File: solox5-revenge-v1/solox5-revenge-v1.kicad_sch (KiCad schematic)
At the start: 36 parts, among them J1 AudioJack4, J2 USB_B_Micro, J3 USB_A, J4 Micro_SD_Card_Det1, SW1 SW_SPDT_MSM, U1 LTC4054ES5-4.2, U2 MIX2018A, U3 AC6965E

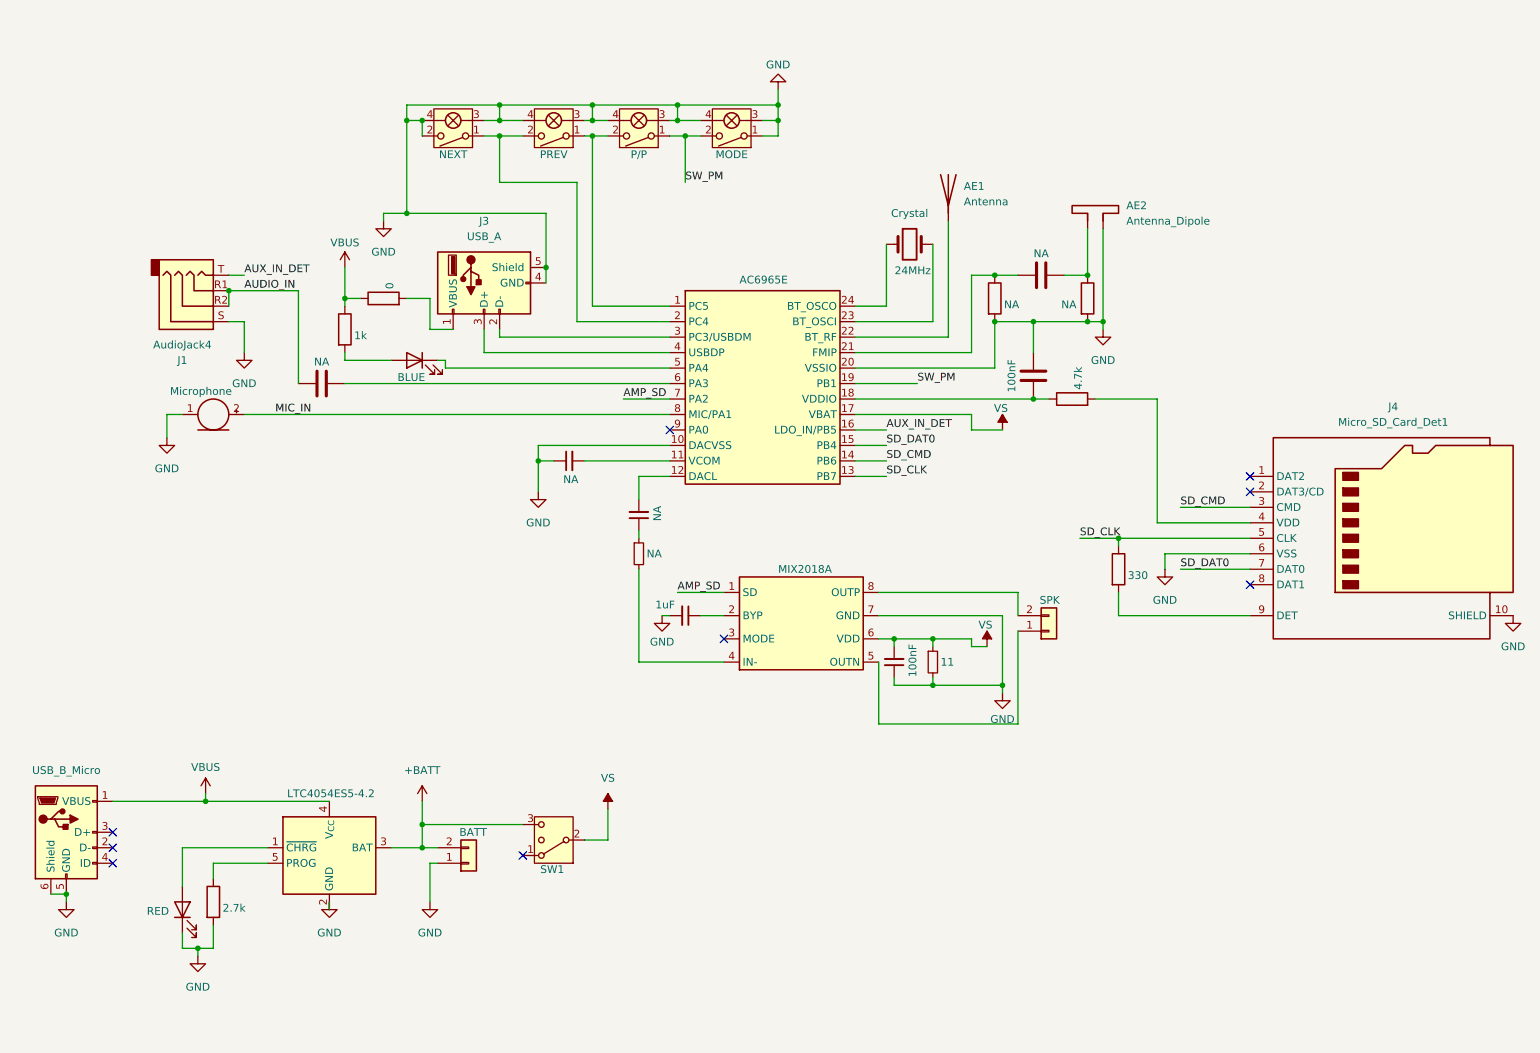
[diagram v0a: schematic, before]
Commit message: [KICAD] Update Sources
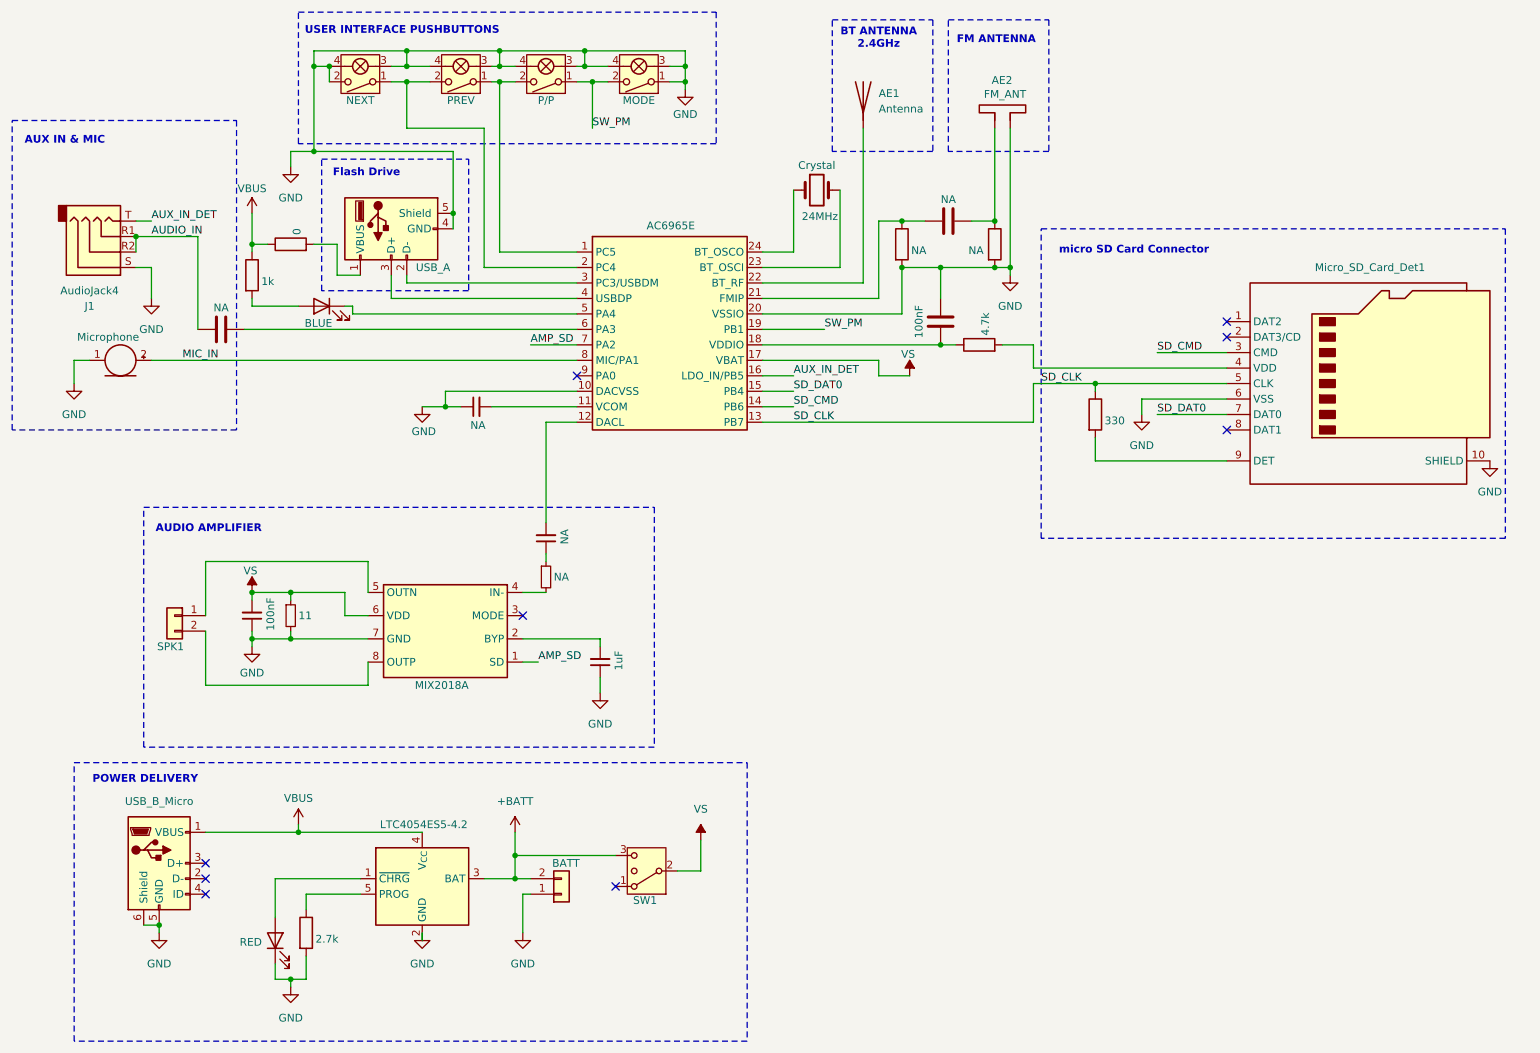
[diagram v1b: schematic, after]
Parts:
- removed C6: 100nF, symbol Device:C_Small
- removed R9: 11, symbol Device:R_Small
- removed SPK: ~, symbol Connector_Generic:Conn_01x02
- added C8: 100nF, symbol Device:C_Small
- added R10: 11, symbol Device:R_Small
- added SPK1: ~, symbol Connector_Generic:Conn_01x02
- AE2: value Antenna_Dipole -> FM_ANT
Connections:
- net GND: now also C7.1, C8.1, R10.2; no longer C7.2
- net VS: now also C8.2, R10.1
- net at U2.2 (BYP): now also C7.2; no longer C7.1
- net at U2.5 (OUTN): now also SPK1.1 (Pin_1)
- net at U2.8 (OUTP): now also SPK1.2 (Pin_2)
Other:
- note added: "AUDIO AMPLIFIER"
- note added: "AUX IN & MIC"
- note added: "BT ANTENNA 2.4GHz"
- note added: "FM ANTENNA"
- note added: "Flash Drive"
- note added: "POWER DELIVERY"
- note added: "USER INTERFACE PUSHBUTTONS"
- note added: "micro SD Card Connector"
- company: (none) -> Helium Labs
- title: (none) -> SOLO X5 Reverse Engineering
- moved on the sheet: 24MHz, AE1, AE2, BATT, BLUE, J1, MODE, NEXT, P/P, PREV, RED, SW1
